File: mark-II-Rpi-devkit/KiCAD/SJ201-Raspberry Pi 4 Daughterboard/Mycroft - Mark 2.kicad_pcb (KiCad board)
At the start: 4 copper layers, 72 x 93 mm, 210 parts, among them J1 Barrel_Jack, J10 Debug Connector, J11 I2S, J2 PVDD Jumper, J3 SPKLEFT, J4 SPKRIGHT, J5 PowerTP, J6 Raspberry_Pi_4, J7 USB_B_Micro, J8 MIC, J9 AudioJack3_Ground_Switch, P1 LED, P2 LED, P3 LED, P4 LED, Q3 AO3415A, Q4 FDV301N, SW1 MuteMic, U1 XL4501E1, U10 SPK0838HT4H-1, U11 SPK0838HT4H-1, U12 NCP303LSN30, U13 CM108B, U3 MAX9744, U4 AZ1117CH-3.3, U5 SN74LVC125APWR, U6 FE1.1s, U7 MP2359, U8 XMOS-XVF3510, U9 AT25SF161 16MBIT, X1 SG-210STF 24M, Y2 12MHz

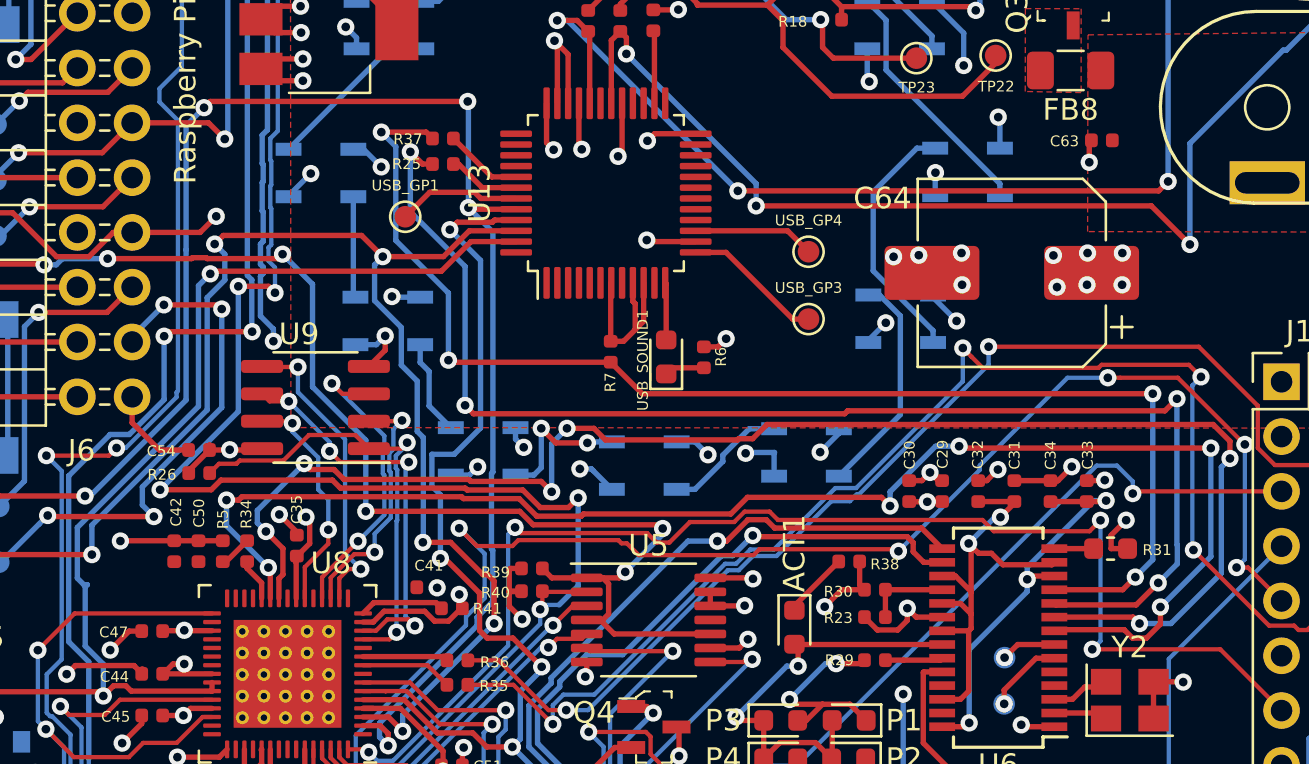
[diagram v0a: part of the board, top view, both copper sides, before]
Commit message: Mark 2 - PCB Files to the printer
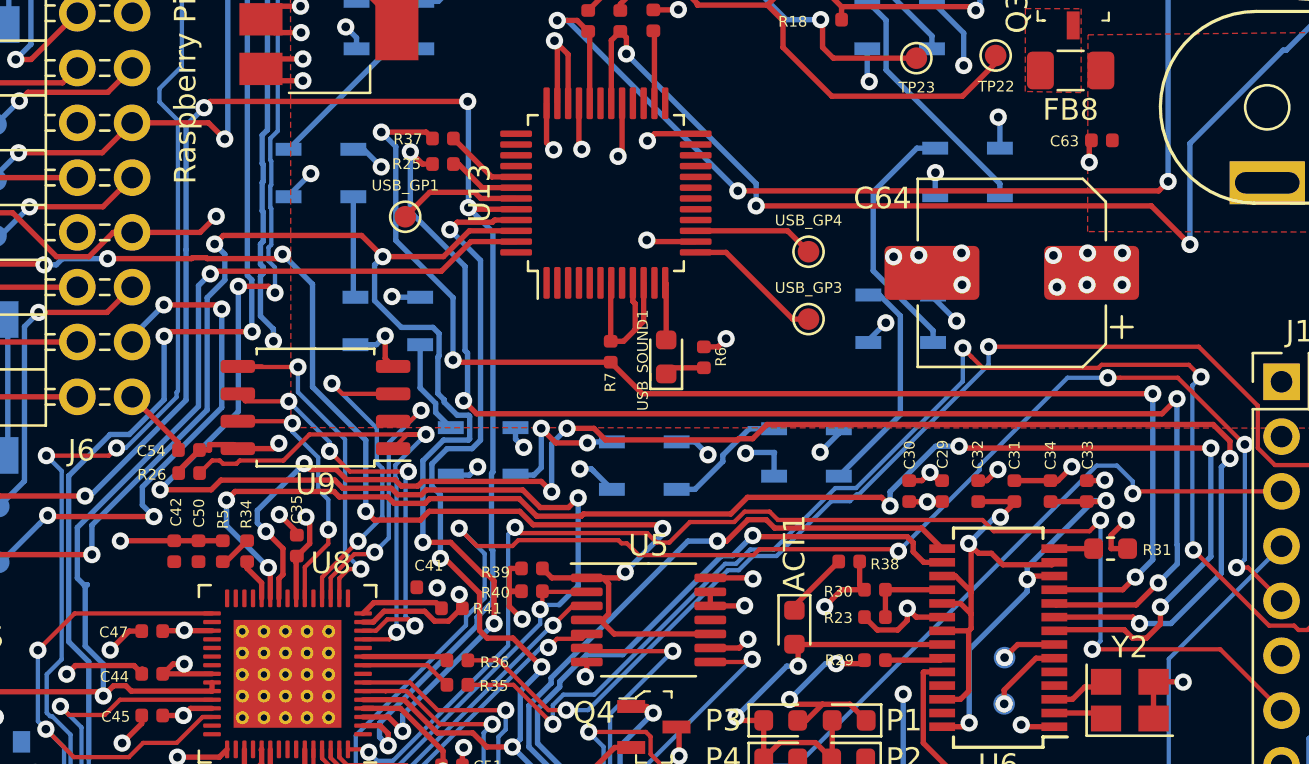
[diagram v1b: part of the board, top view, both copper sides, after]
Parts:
- U9: footprint Package_SO:SOIC-8_3.9x4.9mm_P1.27mm -> Package_SO:SOIC-8_5.23x5.23mm_P1.27mm
- moved C54 0.47 mm to (14.7, 61.7)
- moved R26 0.47 mm to (14.7, 62.8)
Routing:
- net I2S_LRCK: track 81.4 -> 85.1 mm
- net /xmos/QSPI_CS_N: track 21.0 -> 24.6 mm
- net /xmos/QSPI_D0: track 14.4 -> 16.6 mm
- net +3V3: track 86.0 -> 87.4 mm
- net GND: track 238.7 -> 237.6 mm
- net /xmos/QSPI_D3: track 10.7 -> 11.8 mm
- net /xmos/QSPI_D2: track 14.1 -> 15.1 mm
- net /xmos/QSPI_CLK: track 18.9 -> 19.8 mm
- net /xmos/QSPI_D1: track 11.7 -> 12.4 mm
